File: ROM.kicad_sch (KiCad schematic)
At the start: 6 parts, among them U2 SST39SF040, U28 SST39SF040, U4 74LVC245AD

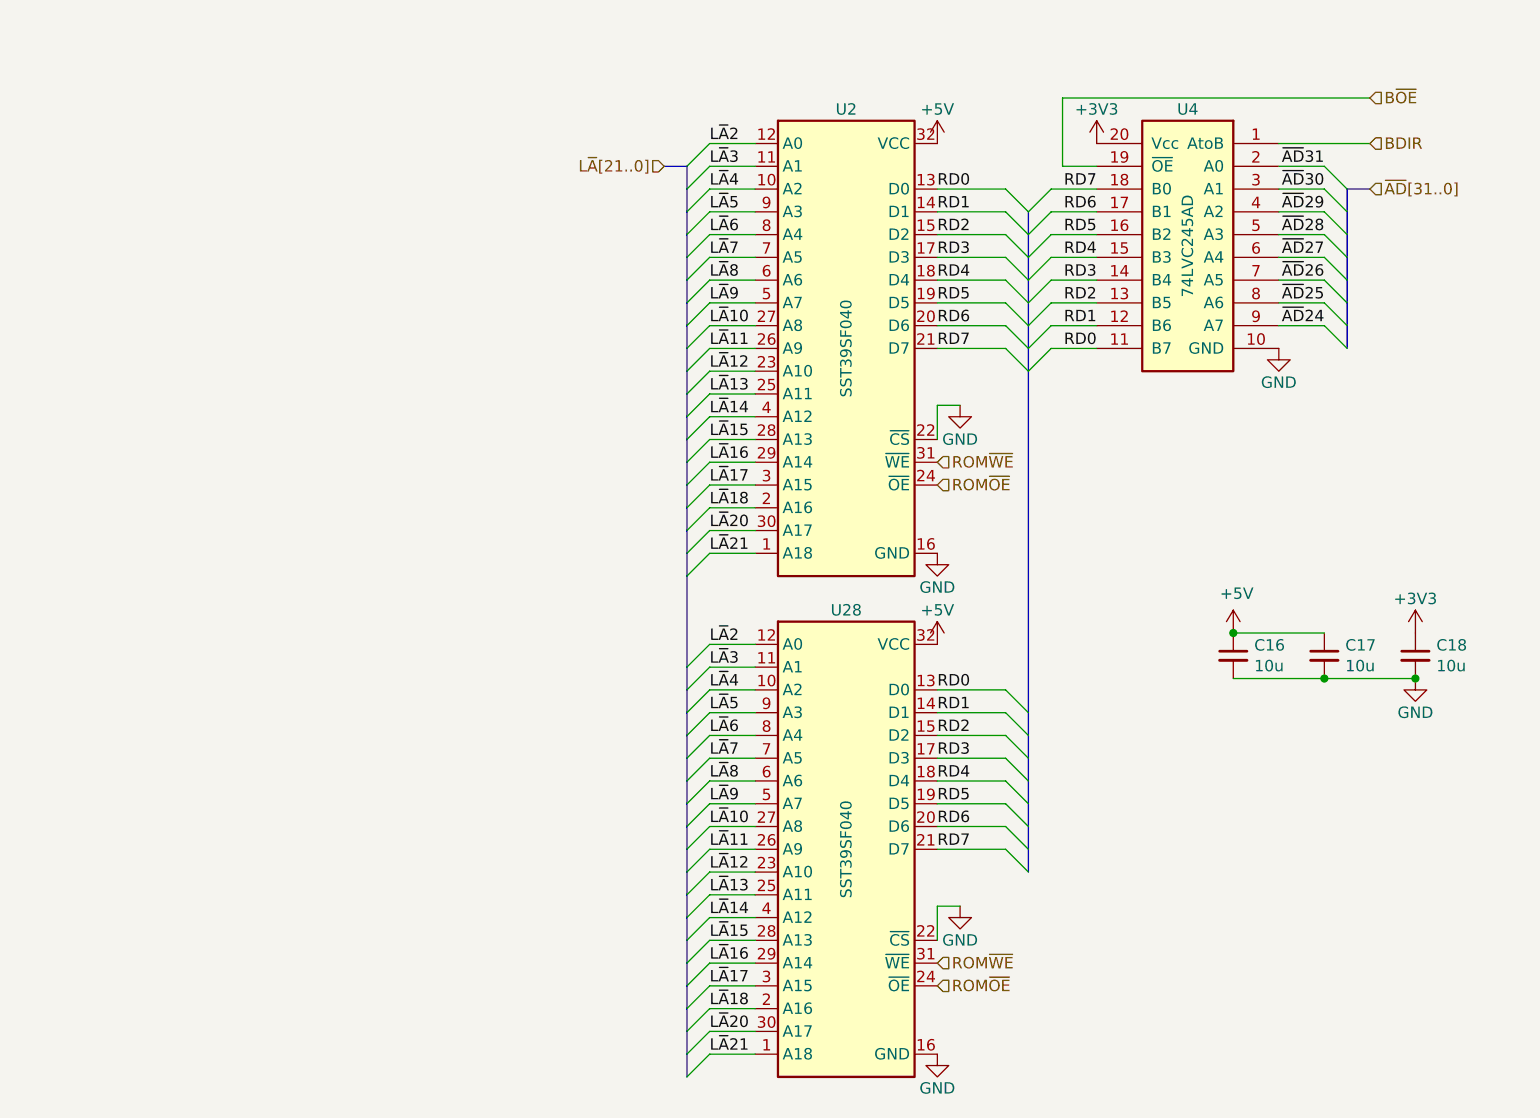
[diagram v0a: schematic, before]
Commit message: work on FPGA
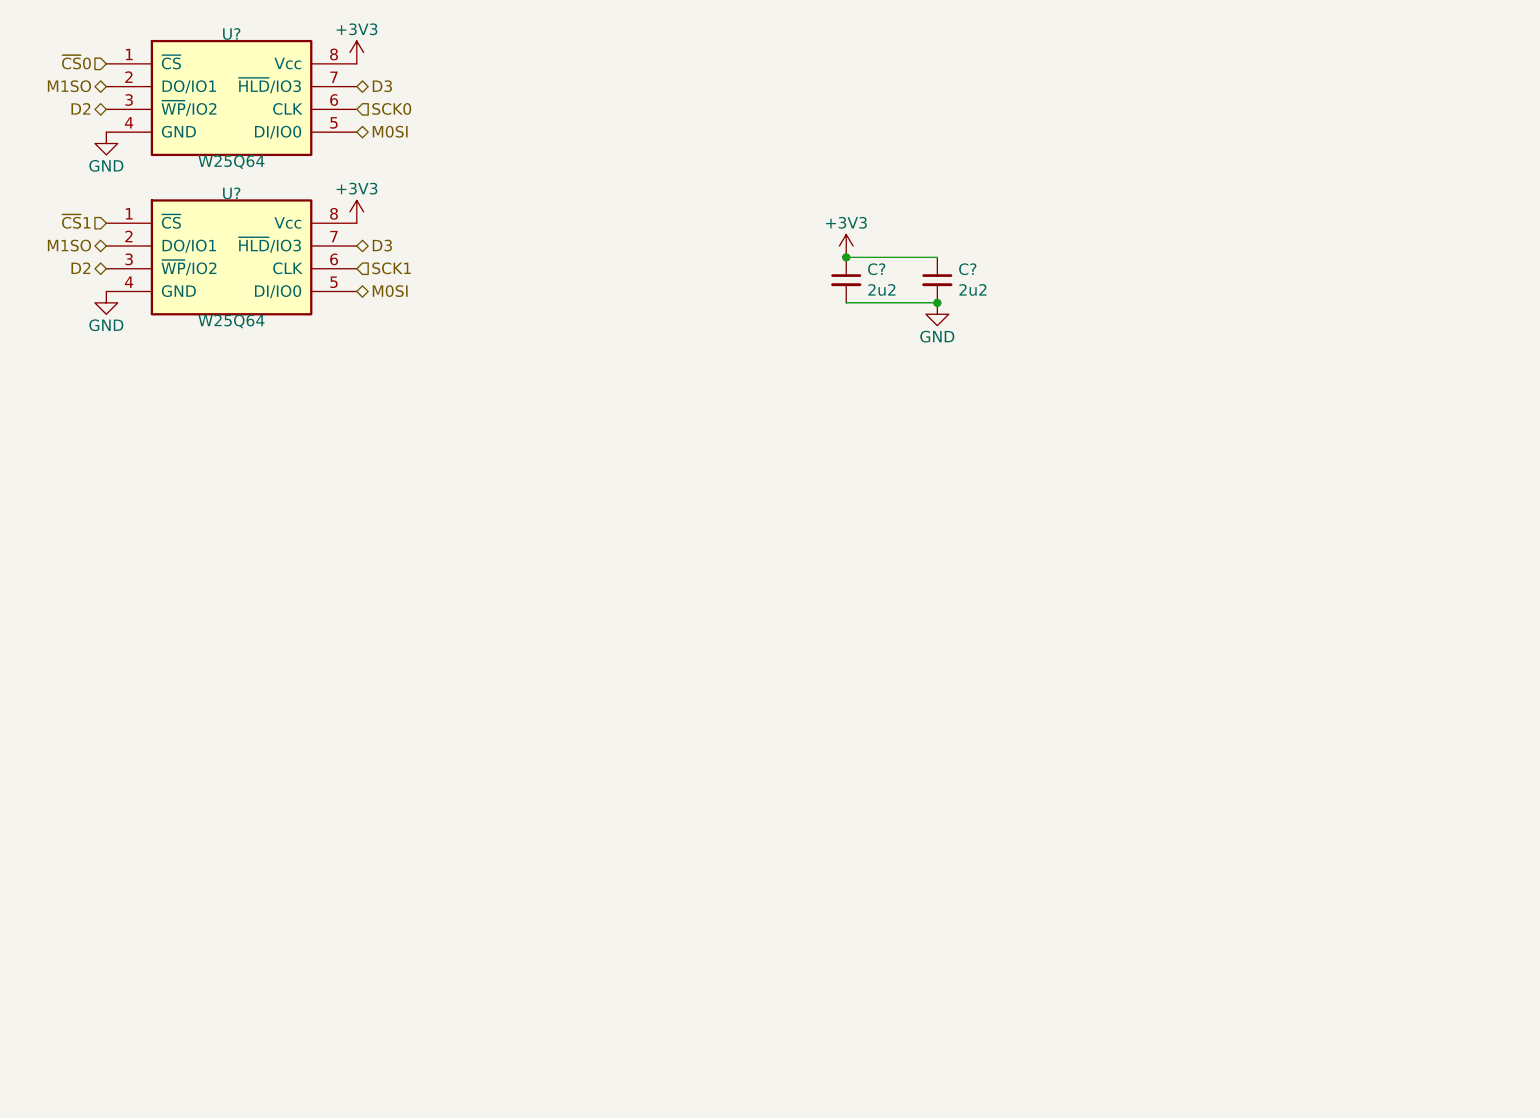
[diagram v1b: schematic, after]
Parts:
- removed C16, C17, C18: 10u, stdpads:C_0805, symbol Device:C_Small
- removed U2: SST39SF040, stdpads:PLCC-32_SMDSocket, symbol GW_RAM:Flash-512Kx8-PLCC-32
- removed U28: SST39SF040, Package_DIP:DIP-32_W15.24mm_Socket_LongPads, symbol GW_RAM:Flash-512Kx8-PLCC-32
- removed U4: 74LVC245AD, stdpads:SOIC-20W_7.5mm, symbol GW_Logic:74245
- added C? (x2): 2u2, stdpads:C_0603, symbol Device:C_Small
- added U? (x2): W25Q64, stdpads:stdpads:SOIC-8_5.3mm, symbol GW_RAM:SPIFlash-SO-8
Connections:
- net +3V3: now also C?.1, C?.1, U?.8 (Vcc), U?.8 (Vcc)
- net GND: now also C?.2, C?.2, U?.4 (GND), U?.4 (GND)
- new net D2: U?.3 (~{WP}/IO2), U?.3 (~{WP}/IO2)
- new net D3: U?.7 (~{HLD}/IO3), U?.7 (~{HLD}/IO3)
- new net M0SI: U?.5 (DI/IO0), U?.5 (DI/IO0)
- new net M1SO: U?.2 (DO/IO1), U?.2 (DO/IO1)
- new net SCK0: U?.6 (CLK)
- new net SCK1: U?.6 (CLK)
- new net ~{CS}0: U?.1 (~{CS})
- new net ~{CS}1: U?.1 (~{CS})
